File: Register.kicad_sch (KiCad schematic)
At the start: 74 parts, among them U1 74LS173, U10 74LS245, U11 74LS245, U12 74LS245, U2 74LS173, U3 74LS173, U4 74LS173, U5 74LS173, U6 74LS173, U7 74LS173, U8 74LS173, U9 74LS245

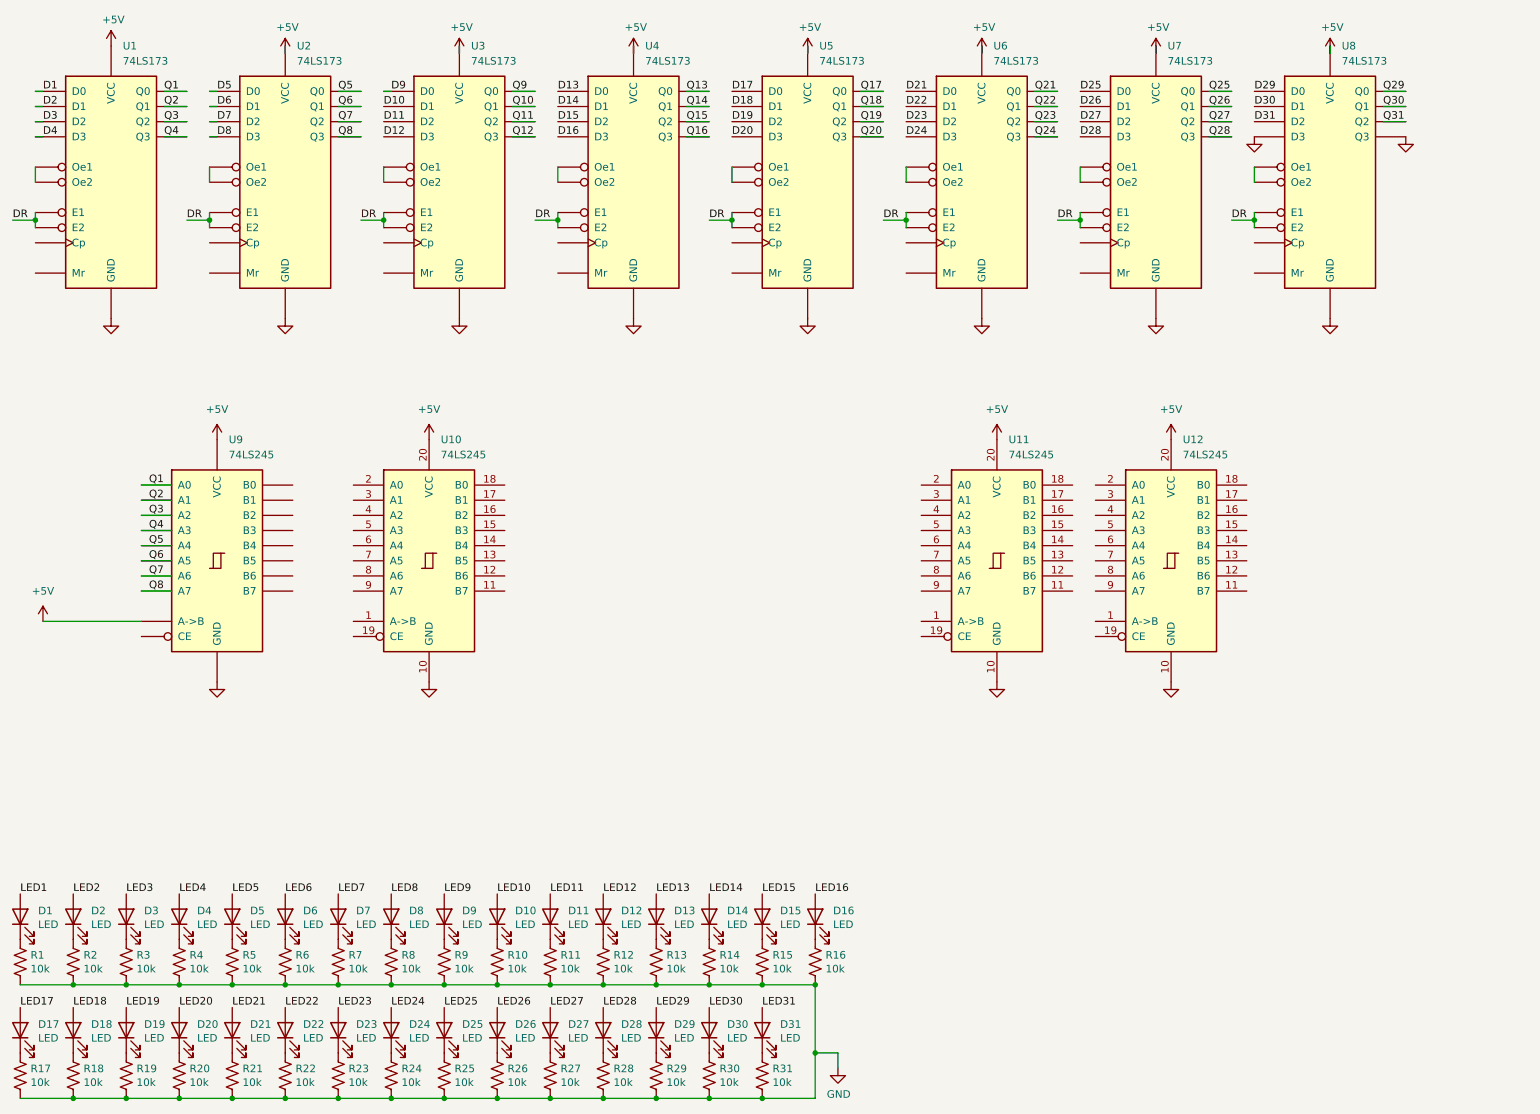
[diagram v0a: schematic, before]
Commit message: Connect and organize Q lines
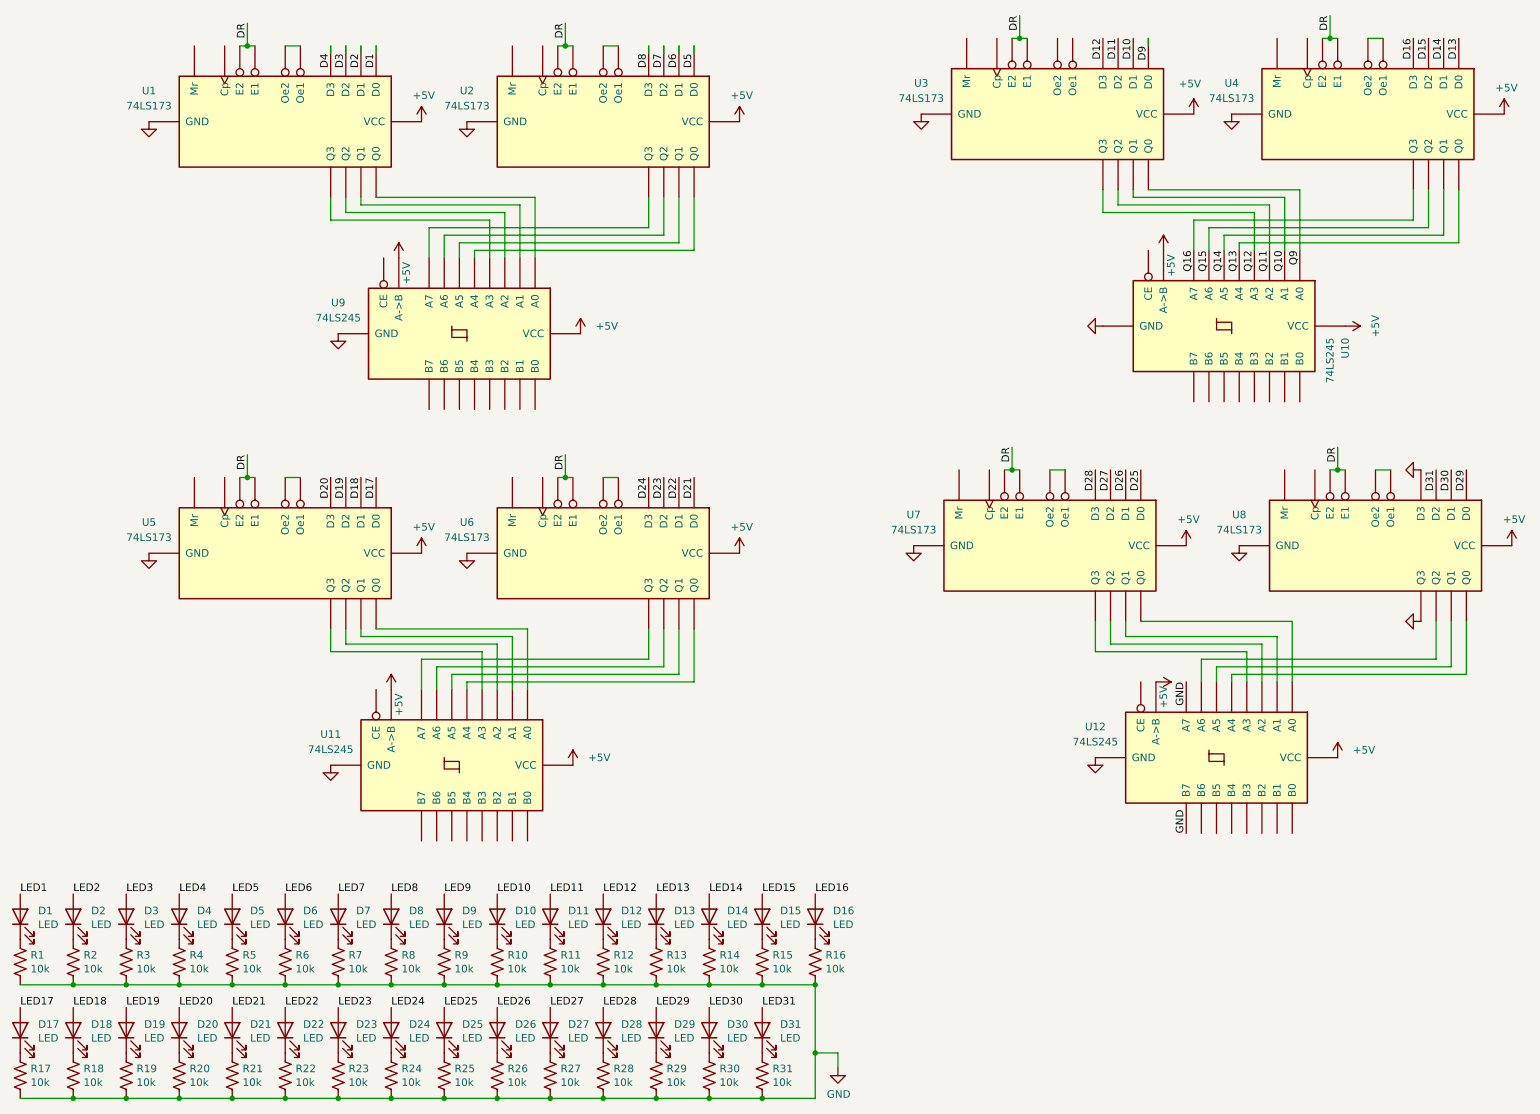
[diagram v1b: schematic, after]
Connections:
- net Q17 is gone; now on an unnamed net: U5.3 (Q0)
- net Q18 is gone; now on an unnamed net: U5.4 (Q1)
- net Q19 is gone; now on an unnamed net: U5.5 (Q2)
- net Q20 is gone; now on an unnamed net: U5.6 (Q3)
- net Q21 is gone; now on an unnamed net: U6.3 (Q0)
- net Q22 is gone; now on an unnamed net: U6.4 (Q1)
- net Q23 is gone; now on an unnamed net: U6.5 (Q2)
- net Q24 is gone; now on an unnamed net: U6.6 (Q3)
- net Q25 is gone; now on an unnamed net: U7.3 (Q0)
- net Q26 is gone; now on an unnamed net: U7.4 (Q1)
- net Q27 is gone; now on an unnamed net: U7.5 (Q2)
- net Q28 is gone; now on an unnamed net: U7.6 (Q3)
- net Q29 is gone; now on an unnamed net: U8.3 (Q0)
- net Q30 is gone; now on an unnamed net: U8.4 (Q1)
- net Q31 is gone; now on an unnamed net: U8.5 (Q2)
- net +5V: now also U10.1 (A->B), U11.1 (A->B), U12.1 (A->B)
- net GND: now also U12.11 (B7), U12.9 (A7)
- net Q10: now also U10.3 (A1)
- net Q11: now also U10.4 (A2)
- net Q12: now also U10.5 (A3)
- net Q13: now also U10.6 (A4)
- net Q14: now also U10.7 (A5)
- net Q15: now also U10.8 (A6)
- net Q16: now also U10.9 (A7)
- net Q9: now also U10.2 (A0)
- net at U3.1 (Oe1): no longer U3.2 (Oe2)
- net Q1: no longer names the net of U1.3 (Q0), U9.2 (A0)
- net Q2: no longer names the net of U1.4 (Q1), U9.3 (A1)
- net Q3: no longer names the net of U1.5 (Q2), U9.4 (A2)
- net Q4: no longer names the net of U1.6 (Q3), U9.5 (A3)
- net Q5: no longer names the net of U2.3 (Q0), U9.6 (A4)
- net Q6: no longer names the net of U2.4 (Q1), U9.7 (A5)
- net Q7: no longer names the net of U2.5 (Q2), U9.8 (A6)
- net Q8: no longer names the net of U2.6 (Q3), U9.9 (A7)
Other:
- moved on the sheet: U1, U2, U3, U4, U5, U6, U7, U8, U9
